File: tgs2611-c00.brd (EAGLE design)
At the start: 25.4 x 17.8 mm, 18 parts, among them J1 3.5mm, J2 M20-9980346, J3 TGS2611-C00, U1 INA219BIDCNT

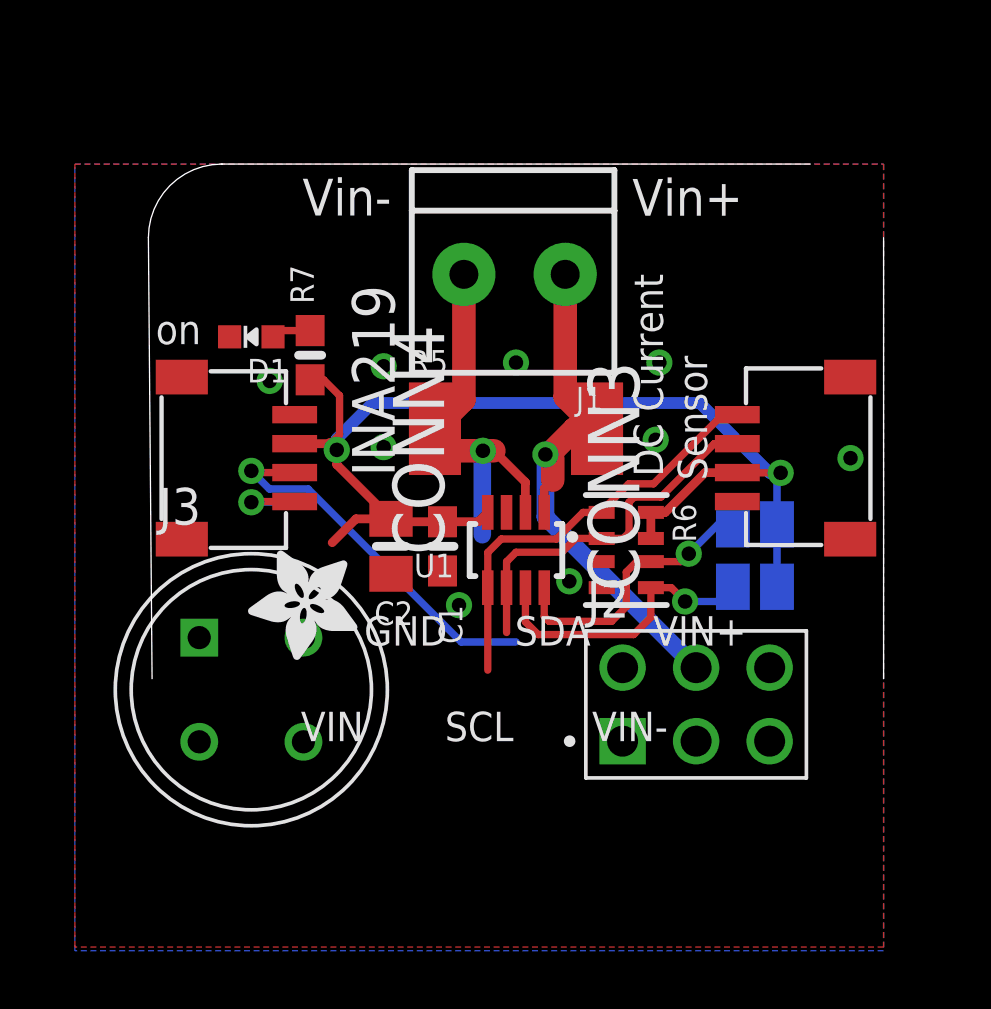
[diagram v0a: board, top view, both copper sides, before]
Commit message: methane PCBs added
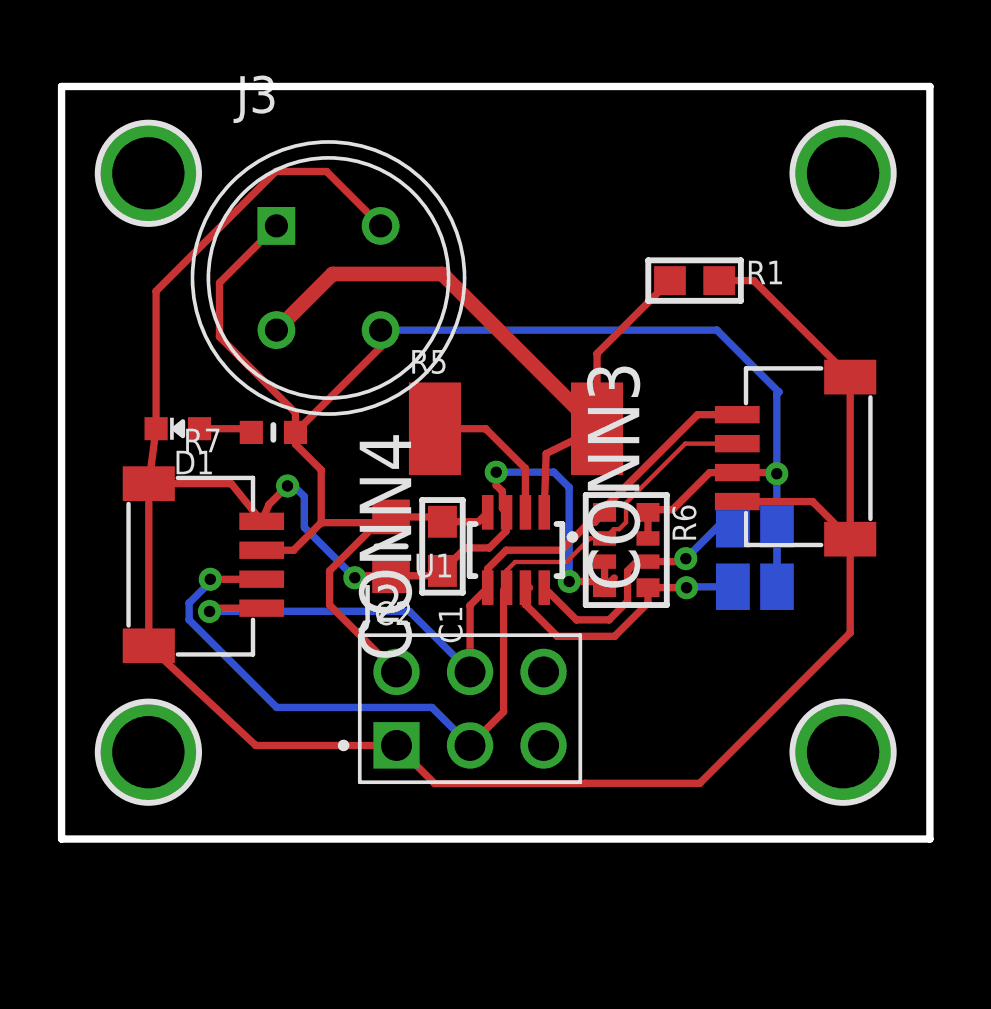
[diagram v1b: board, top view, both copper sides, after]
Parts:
- removed J1: 3.5mm, microbuilder:TERMBLOCK_1X2-3.5MM
- removed U$29: (no value), microbuilder:ADAFRUIT_3.5MM
- removed U$30: (no value), microbuilder:PCBFEAT-REV-040
- removed U$31, U$32: (no value), silks:STEMMAQT
- added R1: 10K, microbuilder:0603
- added U$1, U$6, U$7, U$8: MOUNTINGHOLE2.5, microbuilder:MOUNTINGHOLE_2.5_PLATED
- C1: device microbuilder:0603-NO -> microbuilder:0603
- C2: device microbuilder:0805-NO -> microbuilder:_0805MP
- R7: device microbuilder:0603-NO -> microbuilder:_0603MP
- moved J3 14.5 mm to (6.22, 16.4)
- moved J2 7.81 mm to (11.1, 1.50)
- moved D1 4.07 mm to (1.02, 11.2)
- moved CONN4 3.86 mm to (1.40, 6.48)
- moved R7 2.95 mm to (4.32, 11.0), turned to 180 degrees
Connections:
- removed net VC+: J3.3
- removed net VC-: J3.2
- net GND: now also J2.1, J3.4, R1.2
- net SCL: now also J2.4
- net SDA: now also J2.3
- net VCC: now also J2.2, J3.1, J3.3
- net VIN+: now also J3.2, R1.1; no longer J1.2
- net VIN-: no longer J1.1
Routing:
- net GND: track 0.00 -> 97.1 mm, vias 9 -> 4
- net VCC: track 40.8 -> 59.9 mm, vias 2 -> 1
- net VIN-: track 14.0 -> 5.21 mm, vias 1 -> 0
- net SCL: track 18.0 -> 26.5 mm
- net SDA: track 25.8 -> 32.2 mm
- net VIN+: track 19.9 -> 24.2 mm, vias 1 -> 0
- net ADDR0: track 10.2 -> 9.37 mm
- net ADDR1: track 9.67 -> 8.96 mm
- removed copper zone on layer 1, net GND
- removed copper zone on layer 16, net GND
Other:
- board size 25.4 x 17.8 mm -> 30 x 26 mm
- board text removed: "A0"
- board text removed: "A1"
- board text removed: "Bus Voltage: 0-26V Max Current: ±3.2A Def I2C Addr 0x40"
- board text removed: "DC Current"
- board text removed: "DC Current Monitor"
- board text removed: "GND"
- board text removed: "I2C Addr"
- board text removed: "INA219"
- board text removed: "SCL"
- board text removed: "SDA"
- board text removed: "Sensor"
- board text removed: "VIN"
- board text removed: "VIN+"
- board text removed: "VIN-"
- board text removed: "VLogic/Vcc: 3-5VDC"
- board text removed: "Vin+"
- board text removed: "Vin-"
- board text removed: "on"
